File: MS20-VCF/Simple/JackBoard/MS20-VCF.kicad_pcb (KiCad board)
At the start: 2 copper layers, 60 x 110 mm, 33 parts, among them J11 Conn_JackBoard, J12 Conn_JackBoard, J13 FilterCV2, J14 FilterIn2, J15 FilterOut2, J3 Conn_JackBoard, J4 Conn_JackBoard, J6 FilterCV1, J7 FilterIn1, J8 FilterOut1, SW1 Hpass/Lpass Switch, SW2 Bandpass, SW3 Hpass/Lpass Switch

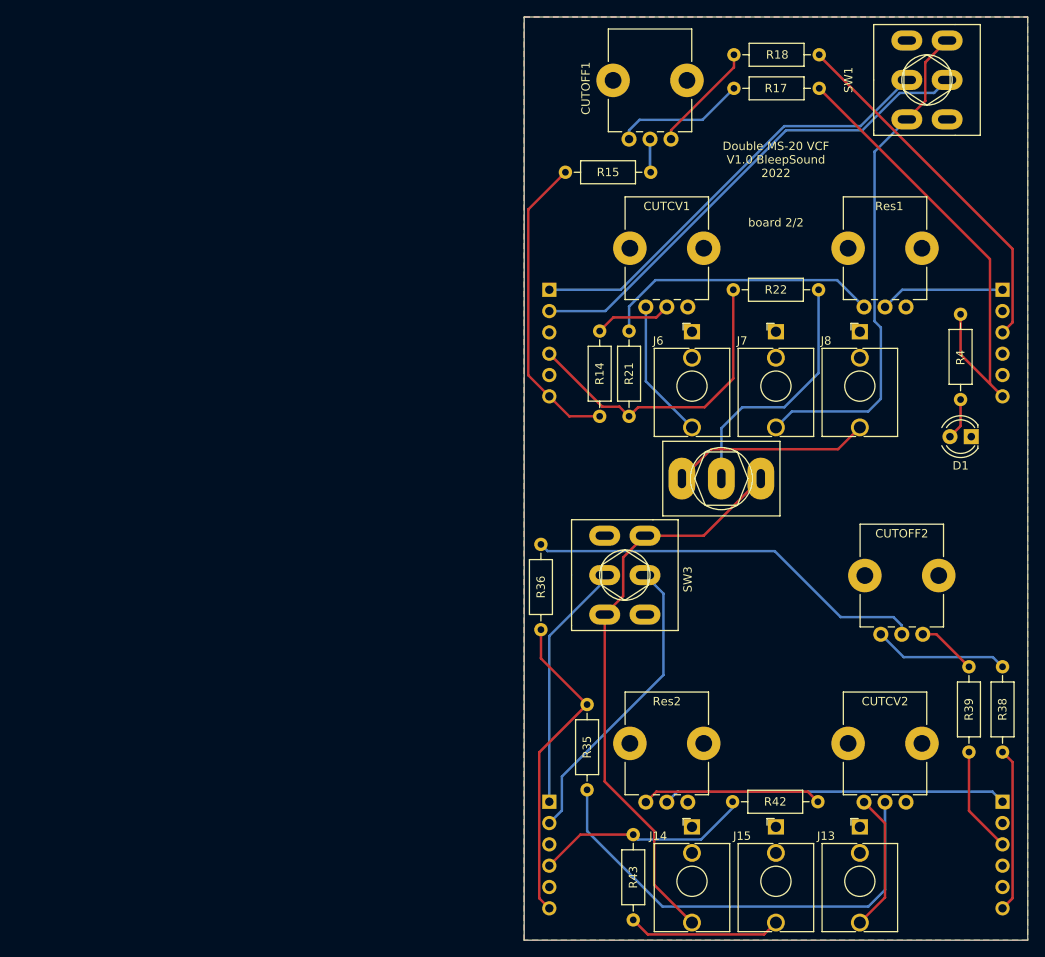
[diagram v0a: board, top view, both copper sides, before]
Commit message: update gerber
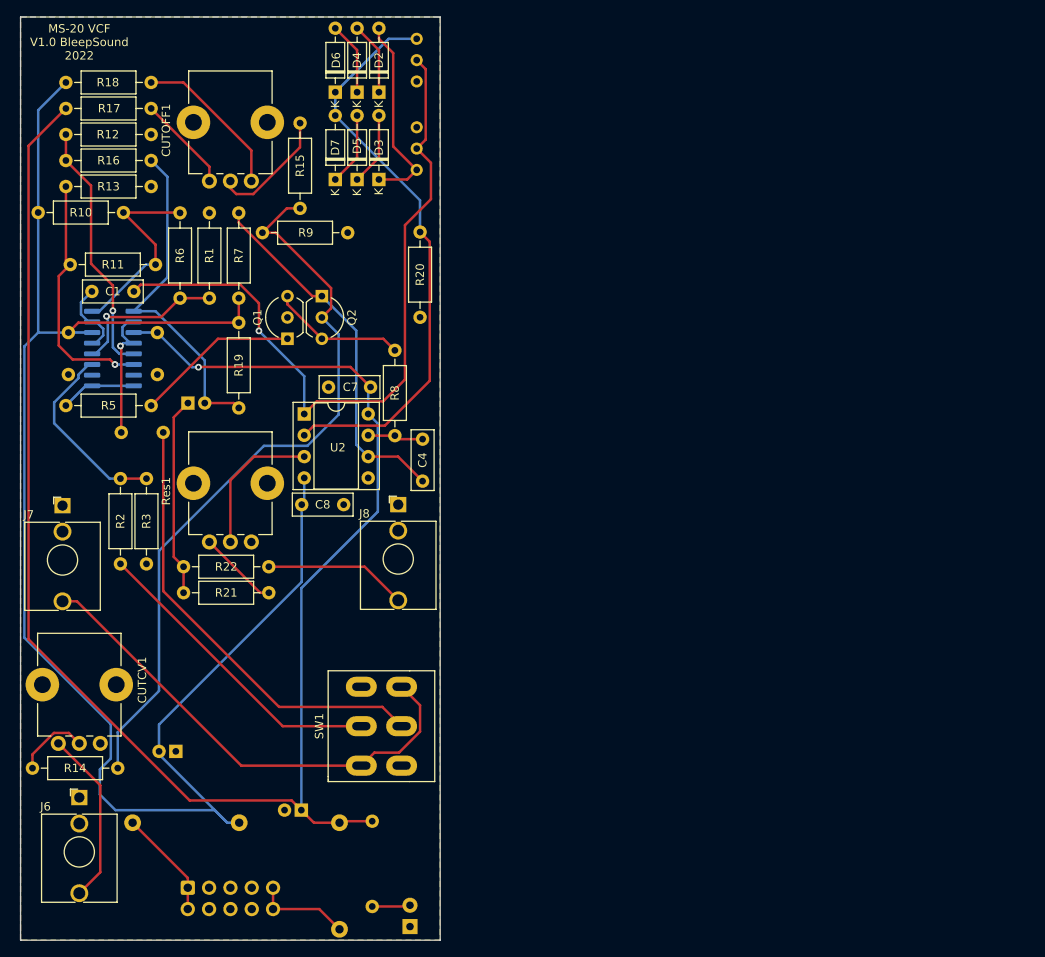
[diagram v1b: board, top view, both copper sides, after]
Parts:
- removed CUTCV2, CUTOFF2, Res2: 100k, Potentiometer_THT:Potentiometer_Bourns_PTV09A-1_Single_Vertical
- removed J11, J12, J3, J4: Conn_JackBoard, Connector_PinHeader_2.54mm:PinHeader_1x06_P2.54mm_Vertical
- removed J13: FilterCV2, Connector_Audio:Jack_3.5mm_QingPu_WQP-PJ398SM_Vertical_CircularHoles
- removed J14: FilterIn2, Connector_Audio:Jack_3.5mm_QingPu_WQP-PJ398SM_Vertical_CircularHoles
- removed J15: FilterOut2, Connector_Audio:Jack_3.5mm_QingPu_WQP-PJ398SM_Vertical_CircularHoles
- removed R35: 82k, Resistor_THT:R_Axial_DIN0207_L6.3mm_D2.5mm_P10.16mm_Horizontal
- removed R36: 100k, Resistor_THT:R_Axial_DIN0207_L6.3mm_D2.5mm_P10.16mm_Horizontal
- removed R38: 33k, Resistor_THT:R_Axial_DIN0207_L6.3mm_D2.5mm_P10.16mm_Horizontal
- removed R39: 56k, Resistor_THT:R_Axial_DIN0207_L6.3mm_D2.5mm_P10.16mm_Horizontal
- removed R42, R43: 1k, Resistor_THT:R_Axial_DIN0207_L6.3mm_D2.5mm_P10.16mm_Horizontal
- removed SW2: Bandpass, Synth:SW_Toggle_Blue_wSlots
- removed SW3: Hpass/Lpass Switch, Synth:SW_DPDT_Toggle
- added C1: 1nF, Capacitor_THT:C_Disc_D7.0mm_W2.5mm_P5.00mm, F.Cu at (43.5, 69.2)
- added C10: 100nF, Capacitor_THT:C_Disc_D7.0mm_W2.5mm_P5.00mm, B.Cu at (40.7, 79.1)
- added C2: 10µ, Capacitor_THT:CP_Radial_D5.0mm_P2.00mm, B.Cu at (68.5, 131.0)
- added C3: 10µ, Capacitor_THT:CP_Radial_D5.0mm_P2.00mm, B.Cu at (53.5, 124.0)
- added C4: 1nF, Capacitor_THT:C_Disc_D7.0mm_W2.5mm_P5.00mm, F.Cu at (82.9, 86.8)
- added C5: 1nF, Capacitor_THT:C_Disc_D7.0mm_W2.5mm_P5.00mm, B.Cu at (47.0, 86.0)
- added C6: 10µF, Capacitor_THT:CP_Radial_D5.0mm_P2.00mm, B.Cu at (54.9, 82.5)
- added C7: 100nF, Capacitor_THT:C_Disc_D7.0mm_W2.5mm_P5.00mm, F.Cu at (76.7, 80.6)
- added C8: 100nF, Capacitor_THT:C_Disc_D7.0mm_W2.5mm_P5.00mm, F.Cu at (73.5, 94.6)
- added C9: 100nF, Capacitor_THT:C_Disc_D7.0mm_W2.5mm_P5.00mm, B.Cu at (51.3, 74.1)
- added D2: 1N4148, Diode_THT:D_DO-35_SOD27_P7.62mm_Horizontal, F.Cu at (77.7, 45.5)
- added D3: 1N4148, Diode_THT:D_DO-35_SOD27_P7.62mm_Horizontal, F.Cu at (77.7, 55.9)
- added D4: 1N4148, Diode_THT:D_DO-35_SOD27_P7.62mm_Horizontal, F.Cu at (75.1, 45.5)
- added D5: 1N4148, Diode_THT:D_DO-35_SOD27_P7.62mm_Horizontal, F.Cu at (75.1, 55.9)
- added D6: 1N4148, Diode_THT:D_DO-35_SOD27_P7.62mm_Horizontal, F.Cu at (72.5, 45.5)
- added D7: 1N4148, Diode_THT:D_DO-35_SOD27_P7.62mm_Horizontal, F.Cu at (72.5, 55.9)
- added FB1: 10R, Inductor_THT:L_Axial_L9.5mm_D4.0mm_P12.70mm_Horizontal_Fastron_SMCC, B.Cu at (73.0, 132.5)
- added FB2: 10R, Inductor_THT:L_Axial_L9.5mm_D4.0mm_P12.70mm_Horizontal_Fastron_SMCC, B.Cu at (61.0, 132.5)
- added J5: Power Input, Connector_IDC:IDC-Header_2x05_P2.54mm_Vertical, B.Cu at (54.9, 140.2)
- added Q1: BC559, Package_TO_SOT_THT:TO-92_Inline_Wide, F.Cu at (66.8, 74.8)
- added Q2: BC559, Package_TO_SOT_THT:TO-92_Inline_Wide, F.Cu at (70.9, 69.8)
- added R1: 470, Resistor_THT:R_Axial_DIN0207_L6.3mm_D2.5mm_P10.16mm_Horizontal, F.Cu at (57.5, 59.8)
- added R10: 1.8k, Resistor_THT:R_Axial_DIN0207_L6.3mm_D2.5mm_P10.16mm_Horizontal, F.Cu at (37.1, 59.8)
- added R11: 100k, Resistor_THT:R_Axial_DIN0207_L6.3mm_D2.5mm_P10.16mm_Horizontal, F.Cu at (51.1, 66.0)
- added R12: 470, Resistor_THT:R_Axial_DIN0207_L6.3mm_D2.5mm_P10.16mm_Horizontal, F.Cu at (50.6, 50.5)
- added R13: 470, Resistor_THT:R_Axial_DIN0207_L6.3mm_D2.5mm_P10.16mm_Horizontal, F.Cu at (50.6, 56.7)
- added R16: 100k, Resistor_THT:R_Axial_DIN0207_L6.3mm_D2.5mm_P10.16mm_Horizontal, F.Cu at (40.4, 53.6)
- added R19: 1.8k, Resistor_THT:R_Axial_DIN0207_L6.3mm_D2.5mm_P10.16mm_Horizontal, F.Cu at (61.0, 72.9)
- added R2: 100k, Resistor_THT:R_Axial_DIN0207_L6.3mm_D2.5mm_P10.16mm_Horizontal, F.Cu at (46.9, 101.7)
- added R20: 2.2k, Resistor_THT:R_Axial_DIN0207_L6.3mm_D2.5mm_P10.16mm_Horizontal, F.Cu at (82.6, 72.3)
- added R3: 470, Resistor_THT:R_Axial_DIN0207_L6.3mm_D2.5mm_P10.16mm_Horizontal, F.Cu at (50.0, 101.7)
- added R5: 2.2k, Resistor_THT:R_Axial_DIN0207_L6.3mm_D2.5mm_P10.16mm_Horizontal, F.Cu at (50.6, 82.8)
- added R6: 100k, Resistor_THT:R_Axial_DIN0207_L6.3mm_D2.5mm_P10.16mm_Horizontal, F.Cu at (54.0, 70.0)
- added R7: 100k, Resistor_THT:R_Axial_DIN0207_L6.3mm_D2.5mm_P10.16mm_Horizontal, F.Cu at (61.0, 70.0)
- added R8: 1k, Resistor_THT:R_Axial_DIN0207_L6.3mm_D2.5mm_P10.16mm_Horizontal, F.Cu at (79.6, 76.2)
- added R9: 2.2k, Resistor_THT:R_Axial_DIN0207_L6.3mm_D2.5mm_P10.16mm_Horizontal, F.Cu at (74.0, 62.2)
- added ResLv1: 3.3k, Potentiometer_THT:Potentiometer_Bourns_3386C_Horizontal, B.Cu at (82.2, 44.2)
- added ResVol1: 10k, Potentiometer_THT:Potentiometer_Bourns_3386C_Horizontal, B.Cu at (82.2, 54.7)
- added U1: LM13700, Package_SO:SOIC-16_3.9x9.9mm_P1.27mm, B.Cu at (46.0, 76.0)
- added U2: TL072, Package_DIP:DIP-8_W7.62mm_Socket, F.Cu at (68.8, 83.8)
- CUTCV1, CUTOFF1, Res1: footprint Potentiometer_THT:Potentiometer_Bourns_PTV09A-1_Single_Vertical -> Synth:Pot-bourns-alpha
- D1, R4: moved to B.Cu
- J6, J7, J8: footprint Connector_Audio:Jack_3.5mm_QingPu_WQP-PJ398SM_Vertical_CircularHoles -> Synth:Thonkiconn
- moved SW1 100.8 mm to (78.0, 121.0)
- moved R4 92.5 mm to (76.9, 132.3)
- moved J6 91.7 mm to (42.0, 129.5)
- moved R18 89.8 mm to (40.4, 44.3), turned to 0 degrees
- moved D1 88.8 mm to (81.4, 144.9), turned to 90 degrees
- moved J7 87.5 mm to (40.0, 94.7)
- moved CUTCV1 87.2 mm to (44.5, 123.0)
- moved Res1 82.9 mm to (62.5, 99.0)
- moved R22 73.3 mm to (64.6, 102.0)
- moved R14 71.1 mm to (46.6, 126.0), turned to 180 degrees
- moved R17 69.5 mm to (50.6, 47.4), turned to 180 degrees
- moved J8 58.7 mm to (80.0, 94.6)
- moved R21 53.1 mm to (64.6, 105.1), turned to 180 degrees
- moved CUTOFF1 50.2 mm to (62.5, 56.0)
- moved R15 31.9 mm to (68.3, 59.3), turned to 90 degrees
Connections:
- R22 pad 1: /FilterOut -> /JackOut
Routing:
- net -12V: track 55.8 -> 191.4 mm
- net +12V: track 75.2 -> 200.9 mm, vias 0 -> 1
- net Net-(C1-Pad2): track 0.00 -> 86.2 mm, vias 0 -> 1
- net Net-(D6-Pad1): track 0.00 -> 69.0 mm
- net Filter2In: track 69.0 -> 0.00 mm
- net Net-(CUTCV2-Pad2): track 55.4 -> 0.00 mm
- net /Cutoff: track 36.6 -> 89.0 mm
- net Net-(CUTOFF2-Pad2): track 48.1 -> 0.00 mm
- net Net-(C4-Pad2): track 0.00 -> 43.8 mm
- net /Filtre2/ResOut: track 41.0 -> 0.00 mm
- net Net-(C6-Pad2): track 0.00 -> 40.7 mm
- net /Filtre2/Cutoff: track 38.3 -> 0.00 mm
- net /Filtre2/HPass: track 36.1 -> 0.00 mm
- net Net-(R12-Pad2): track 0.00 -> 30.5 mm, vias 0 -> 1
- net /FilterOut: track 30.2 -> 0.00 mm
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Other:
- board size 60 x 110 mm -> 50 x 110 mm
- board text added: "MS-20 VCF V1.0 BleepSound 2022"
- board text removed: "12HP"
- board text removed: "Double MS-20 VCF V1.0 BleepSound 2022"
- board text removed: "board 2/2"
